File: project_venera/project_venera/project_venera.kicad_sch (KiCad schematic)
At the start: 22 parts, among them IC1 NCV303LSN11T1G, IC2 TC1262-3.3VDBTR, IC3 ATSAMD11D14A-SSUT, J1 0022285034, J2 0022285034, J3 0022285034, J4 0022285034, P1 TC2030-CTX

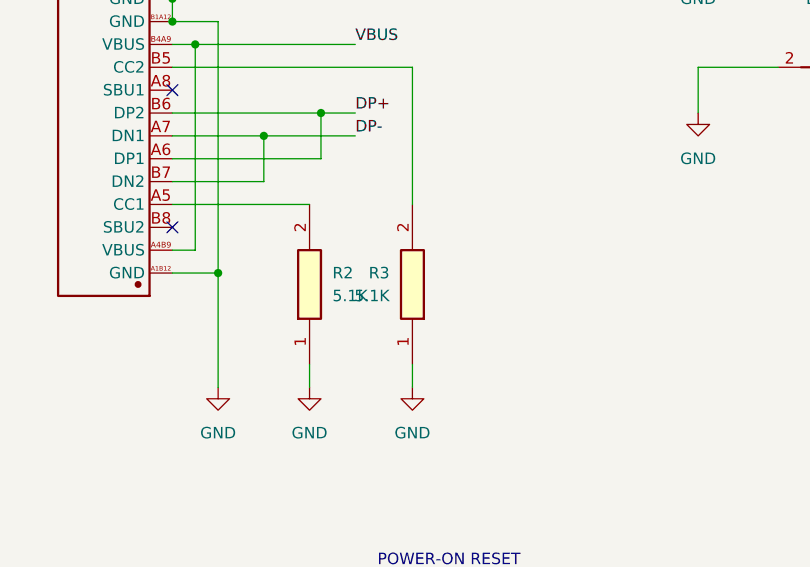
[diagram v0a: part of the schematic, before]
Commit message: update venera hw
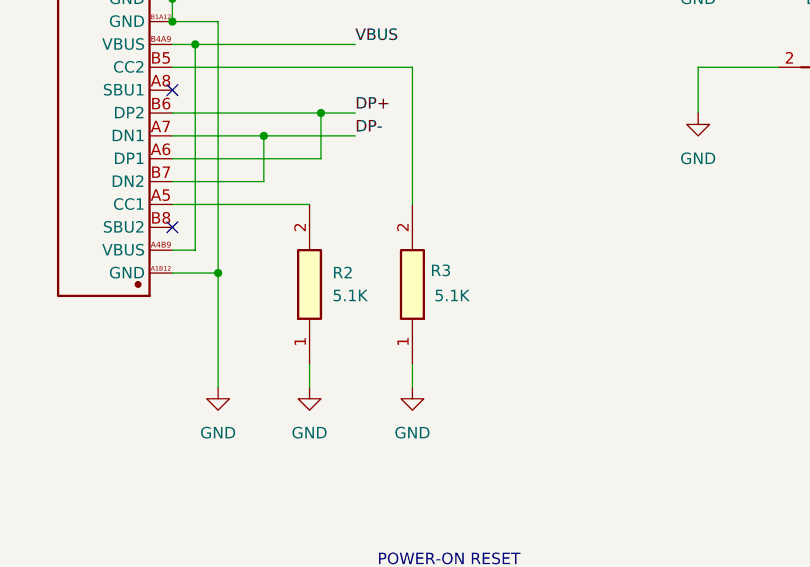
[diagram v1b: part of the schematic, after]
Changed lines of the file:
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@@
 		(dnp no)
 		(property "Reference" "R3"
-			(at 58.42 73.6599 90)
+			(at 65.278 73.406 90)
 			(show_name no)
 			(do_not_autoplace no)
@@
 		)
 		(property "Value" "5.1K"
-			(at 58.42 76.1999 90)
+			(at 67.31 76.2 90)
 			(show_name no)
 			(do_not_autoplace no)
